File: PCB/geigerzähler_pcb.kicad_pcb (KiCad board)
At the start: 2 copper layers, 155 x 40 mm, 98 parts, among them J1 Molex Micro Fit, J2 Debugpins, J3 USB-TYPE-C-018, J4 Femal Connector for LCD I2C b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, Q1 IRLML6402TRPBF, Q2 BCW68, Q3 PBHV8560Z, Q4 MMBT3904, Q5 MMBT3904, SW1 GPIO4, SW2 GPIO5, SW3 Reset, SW4 Boot, SW5 SW_SPDT, U1 TPS631000DRLR, U2 MCP73871-2AA, U3 ESP32-S3-WROOM-1_multi_unit, U4 ICM7555IBAZ

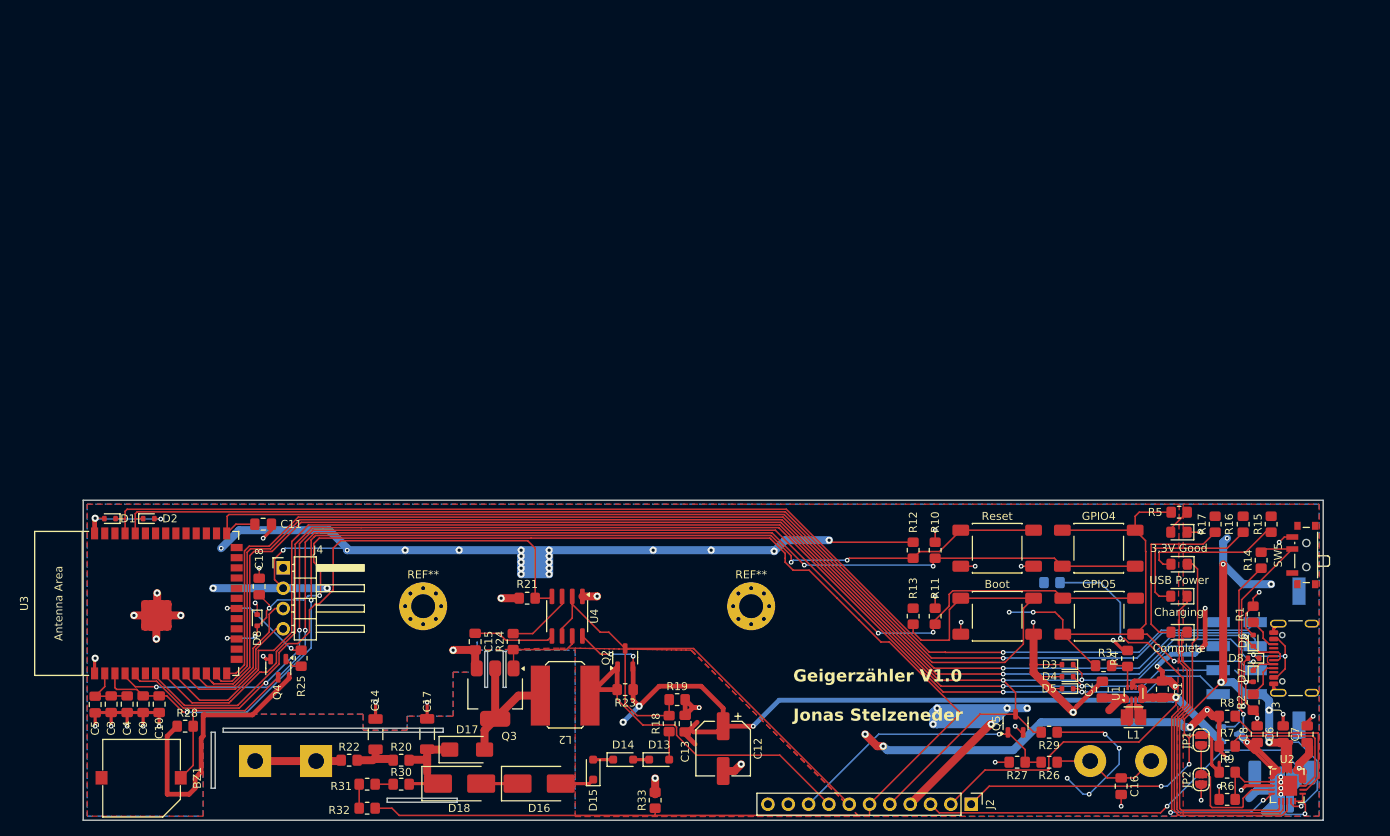
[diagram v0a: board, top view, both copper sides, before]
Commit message: 08.08.2025_v0.2_start
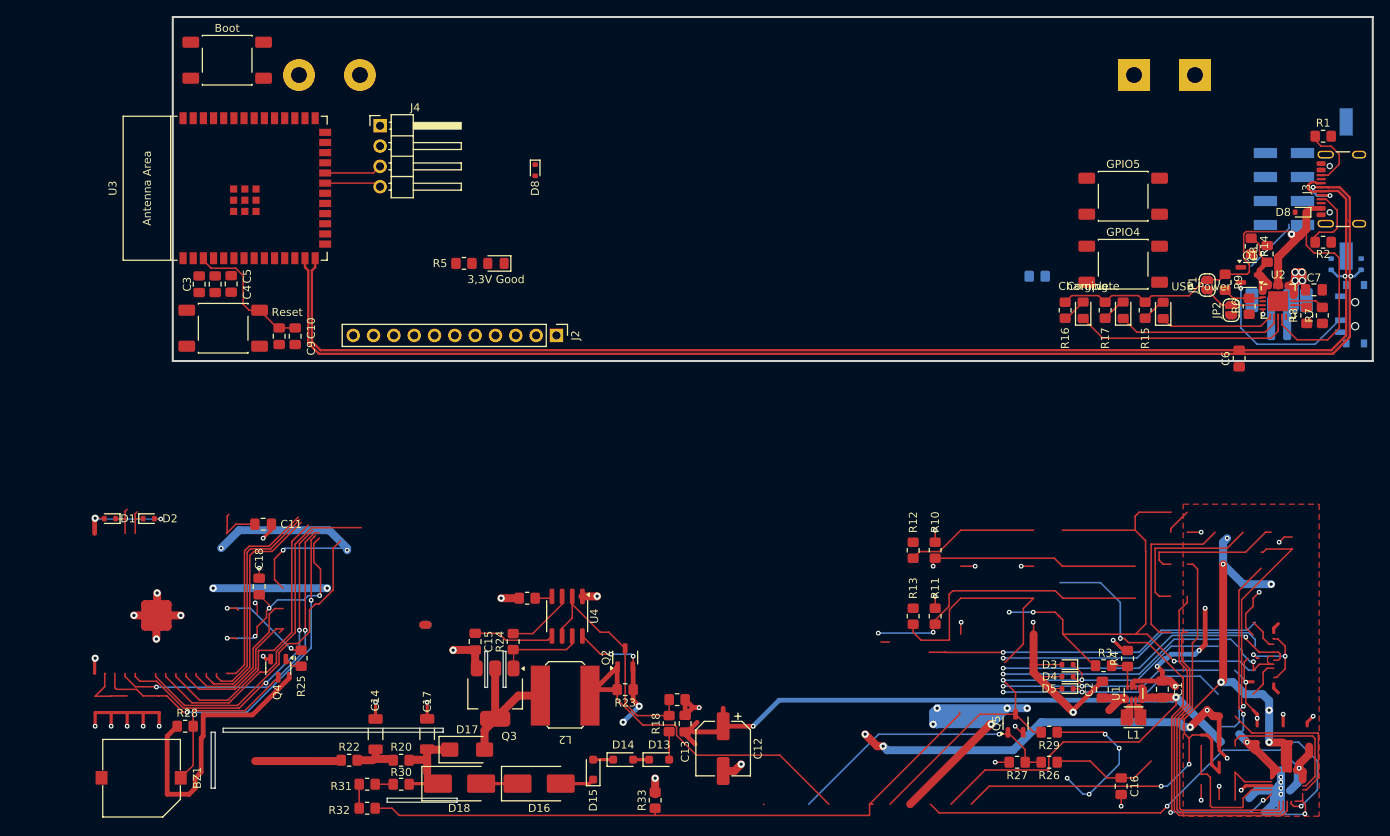
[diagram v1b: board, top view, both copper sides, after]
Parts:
- removed REF** (x2): MountingHole_3mm_Pad_Via, MountingHole:MountingHole_3mm_Pad_Via
- D6, D7, SW5: moved to B.Cu
- Q1: moved to F.Cu
- moved V1 145.4 mm to (209.0, 46.8), turned to 180 degrees
- moved SW4 118.7 mm to (88.0, 45.0)
- moved SW3 100.6 mm to (87.5, 78.5)
- moved R5 94.7 mm to (117.6, 70.4)
- moved D9 91.7 mm to (121.6, 70.4)
- moved J2 78.2 mm to (129.2, 79.4)
- moved D8 66.1 mm to (126.5, 58.8)
- moved R6 61.7 mm to (215.8, 75.8), turned to 90 degrees
- moved R9 61.3 mm to (212.8, 72.8), turned to -90 degrees
- moved U2 60.6 mm to (219.4, 75.1)
- moved R1 60.4 mm to (225.0, 54.5), turned to 0 degrees
- moved C8 60.1 mm to (218.0, 69.2)
- moved BT1 59.1 mm to (219.5, 76.8)
- moved J1 58.9 mm to (220.1, 61.1)
- moved J3 58.9 mm to (228.4, 61.1)
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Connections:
- D3 pad 1: GPIO8 -> GPIO1
- J1 pad 7: GPIO8 -> GPIO1
- Q5 pad 3: GPIO8 -> GPIO1
- R10 pad 1: Net-(U3A-GPIO4) -> Net-(U3A-GPIO10)
- R11 pad 1: Net-(U3A-GPIO5) -> Net-(U3A-GPIO11)
- R21 pad 1: GPIO7 -> GPIO9
- R29 pad 2: GPIO8 -> GPIO1
- SW1 pad 1: Net-(U3A-GPIO4) -> Net-(U3A-GPIO10)
- SW1 pad 3: Net-(U3A-GPIO4) -> Net-(U3A-GPIO10)
- SW2 pad 1: Net-(U3A-GPIO5) -> Net-(U3A-GPIO11)
- SW2 pad 3: Net-(U3A-GPIO5) -> Net-(U3A-GPIO11)
- SW5 pad : (no net) -> GND
- U3 pad 10: I2C_SCL -> unconnected-(U3B-GPIO17/I2C_SCL-Pad10)
- U3 pad 11: I2C_SDA -> unconnected-(U3B-GPIO18/I2C_SDA-Pad11)
- U3 pad 12: GPIO8 -> unconnected-(U3B-GPIO8-Pad12)
- U3 pad 15: unconnected-(U3B-GPIO3/TOUCH3/ADC1_CH2-Pad15) -> Vhigh/100
- U3 pad 17: Vhigh/100 -> GPIO9
- U3 pad 18: unconnected-(U3B-GPIO10/TOUCH10/ADC1_CH9/FSPICS0/FSPIIO4/SUBSPICS0-Pad18) -> Net-(U3A-GPIO10)
- U3 pad 19: unconnected-(U3B-GPIO11/TOUCH11/ADC2_CH0/FSPID/FSPIIO5/SUBSPID-Pad19) -> Net-(U3A-GPIO11)
- U3 pad 21: unconnected-(U3B-GPIO13/TOUCH13/ADC2_CH2/FSPIQ/FSPIIO7/SUBSPIQ-Pad21) -> I2C_SCL
- U3 pad 22: unconnected-(U3B-GPIO14/TOUCH14/ADC2_CH3/FSPIWP/FSPIDQS/SUBSPIWP-Pad22) -> I2C_SDA
- U3 pad 39: unconnected-(U3B-GPIO1-Pad39) -> GPIO1
- U3 pad 4: Net-(U3A-GPIO4) -> unconnected-(U3B-GPIO4-Pad4)
- U3 pad 5: Net-(U3A-GPIO5) -> unconnected-(U3B-GPIO5-Pad5)
- U3 pad 7: GPIO7 -> unconnected-(U3B-GPIO7-Pad7)
- U4 pad 4: GPIO7 -> GPIO9
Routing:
- net GPIO8: track 185.6 -> 29.3 mm, vias 2 -> 0
- net Net-(U3A-GPIO5): track 153.5 -> 0.00 mm, vias 4 -> 0
- net UART0_TX: track 154.3 -> 4.34 mm, vias 1 -> 0
- net Net-(U3A-GPIO4): track 146.1 -> 0.00 mm, vias 4 -> 0
- net (no net): track 0.00 -> 121.4 mm, vias 0 -> 4
- net UART0_RX: track 153.6 -> 37.8 mm
- net Net-(U3A-GPIO0/BOOT): track 141.6 -> 36.9 mm
- net GPIO16/U0CTS: track 159.9 -> 64.7 mm
- net +3.3V: track 325.7 -> 233.7 mm, vias 33 -> 17
- net GPIO15/U0RTS: track 161.2 -> 72.5 mm
- net Vhigh/100: track 196.8 -> 108.2 mm
- net VBUS: track 132.1 -> 212.4 mm, vias 11 -> 13
- net D-: track 164.4 -> 239.1 mm, vias 2 -> 5
- net GPIO7: track 72.2 -> 0.00 mm
- net D+: track 160.2 -> 232.2 mm, vias 2 -> 3
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- removed copper zone on F.Cu, net +3.3V
- removed copper zone on B.Cu, net GND
- removed copper zone on F.Cu, net Vbat_USB
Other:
- board size 155 x 40 mm -> 150 x 98.2 mm
- board text removed: "Geigerzähler V1.0 Jonas Stelzeneder"

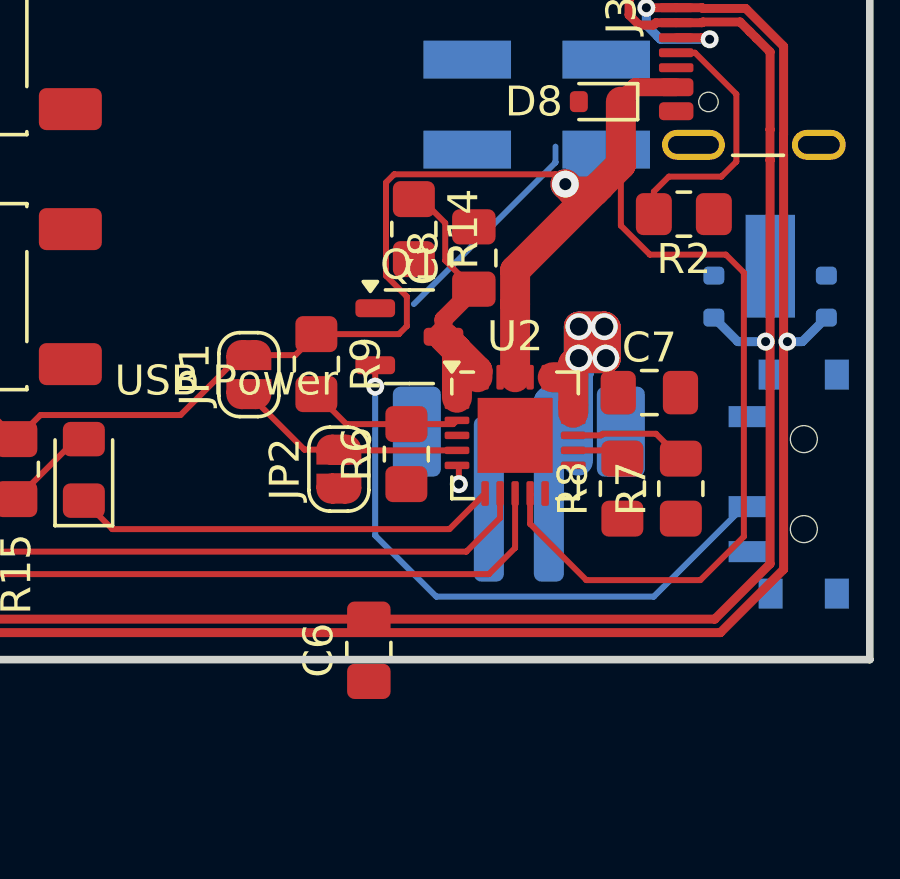
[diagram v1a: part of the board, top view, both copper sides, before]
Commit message: 08.08.2025
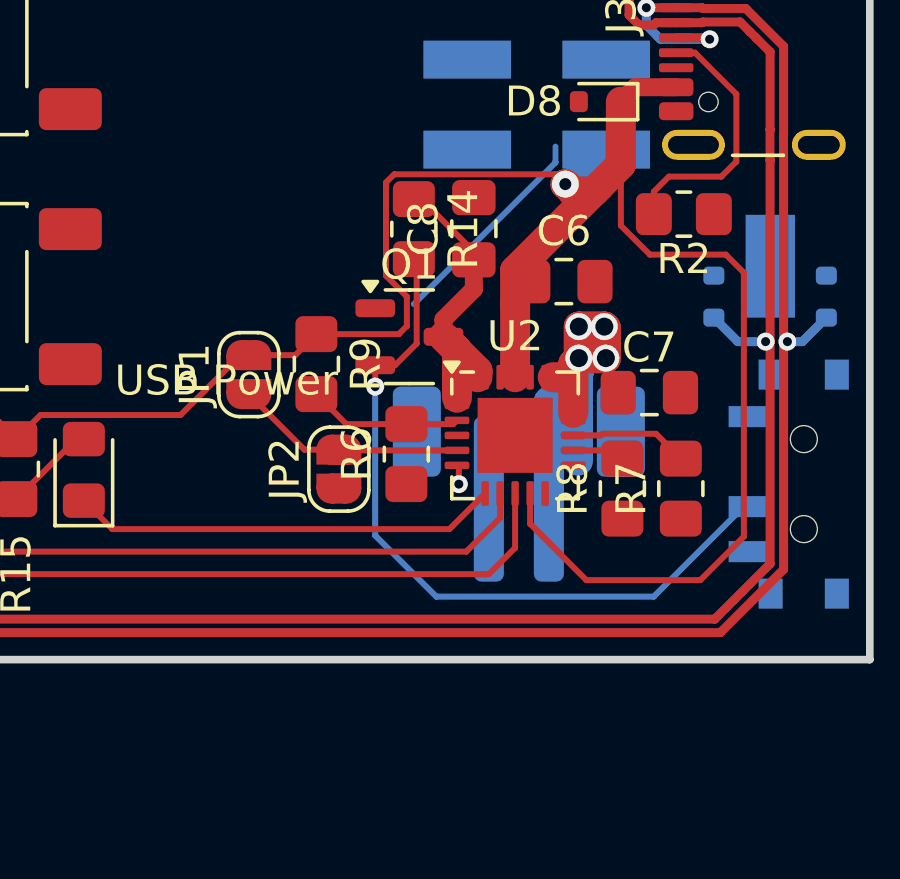
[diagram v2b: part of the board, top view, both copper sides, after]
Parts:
- moved C6 13.9 mm to (221.0, 70.0), turned to 0 degrees
- moved C8 0.98 mm to (218.0, 68.2)
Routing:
- net Net-(Q1-G): track 58.9 -> 63.4 mm
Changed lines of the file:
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@@
 	(footprint "Capacitor_SMD:C_0805_2012Metric_Pad1.18x1.45mm_HandSolder"
 		(layer "F.Cu")
-		(at 218 69.2125 90)
+		(at 218 68.2375 90)
 		(descr "Capacitor SMD 0805 (2012 Metric), square (rectangular) end terminal, IPC-7351 nominal with elongated pad for handsoldering. (Body size source: IPC-SM-782 page 76, https://www.pcb-3d.com/wordpress/wp-content/uploads/ipc-sm-782a_amendment_1_and_2.pdf, https://docs.google.com/spreadsheets/d/1BsfQQcO9C6DZCsRaXUlFlo91Tg2WpOkGARC1WS5S8t0/edit?usp=sharing), generated with kicad-footprint-generator")
 		(tags "capacitor handsolder")
@@
 	(footprint "Capacitor_SMD:C_0805_2012Metric_Pad1.18x1.45mm_HandSolder"
 		(layer "F.Cu")
-		(at 214.5 82.2875 90)
+		(at 221 70)
 		(descr "Capacitor SMD 0805 (2012 Metric), square (rectangular) end terminal, IPC-7351 nominal with elongated pad for handsoldering. (Body size source: IPC-SM-782 page 76, https://www.pcb-3d.com/wordpress/wp-content/uploads/ipc-sm-782a_amendment_1_and_2.pdf, https://docs.google.com/spreadsheets/d/1BsfQQcO9C6DZCsRaXUlFlo91Tg2WpOkGARC1WS5S8t0/edit?usp=sharing), generated with kicad-footprint-generator")
 		(tags "capacitor handsolder")
 		(property "Reference" "C6"
-			(at 0 -1.68 90)
+			(at 0 -1.68 0)
 			(layer "F.SilkS")
 			(effects
@@
 		)
 		(property "Value" "10µF"
-			(at 0 1.68 90)
+			(at 0 1.68 0)
 			(layer "F.Fab")
 			(effects
@@
 		)
 		(property "Datasheet" "https://jlcpcb.com/partdetail/439567-GRM21BR61H106KE43L/C440198"
-			(at 0 0 90)
+			(at 0 0 0)
 			(layer "F.Fab")
 			(hide yes)
@@
 		)
 		(property "Description" "Unpolarized capacitor, small symbol"
-			(at 0 0 90)
+			(at 0 0 0)
 			(layer "F.Fab")
 			(hide yes)
@@
 		)
 		(fp_line
-			(start 1.88 -0.98)
-			(end 1.88 0.98)
+			(start -1.88 -0.98)
+			(end 1.88 -0.98)
 			(stroke
 				(width 0.05)
@@
 		)
 		(fp_line
-			(start -1.88 -0.98)
-			(end 1.88 -0.98)
+			(start -1.88 0.98)
+			(end -1.88 -0.98)
 			(stroke
 				(width 0.05)
@@
 		)
 		(fp_line
-			(start 1.88 0.98)
-			(end -1.88 0.98)
+			(start 1.88 -0.98)
+			(end 1.88 0.98)
 			(stroke
 				(width 0.05)
@@
 		)
 		(fp_line
-			(start -1.88 0.98)
-			(end -1.88 -0.98)
+			(start 1.88 0.98)
+			(end -1.88 0.98)
 			(stroke
 				(width 0.05)
@@
 		)
 		(fp_line
-			(start 1 -0.625)
-			(end 1 0.625)
+			(start -1 -0.625)
+			(end 1 -0.625)
 			(stroke
 				(width 0.1)
@@
 		)
 		(fp_line
-			(start -1 -0.625)
-			(end 1 -0.625)
+			(start -1 0.625)
+			(end -1 -0.625)
 			(stroke
 				(width 0.1)
@@
 		)
 		(fp_line
-			(start 1 0.625)
-			(end -1 0.625)
+			(start 1 -0.625)
+			(end 1 0.625)
 			(stroke
 				(width 0.1)
@@
 		)
 		(fp_line
-			(start -1 0.625)
-			(end -1 -0.625)
+			(start 1 0.625)
+			(end -1 0.625)
 			(stroke
 				(width 0.1)
@@
 		)
 		(fp_text user "${REFERENCE}"
-			(at 0 0 90)
+			(at 0 0 0)
 			(layer "F.Fab")
 			(effects
@@
 		)
 		(pad "1" smd roundrect
-			(at -1.0375 0 90)
+			(at -1.0375 0)
 			(size 1.175 1.45)
 			(layers "F.Cu" "F.Mask" "F.Paste")
@@
 		)
 		(pad "2" smd roundrect
-			(at 1.0375 0 90)
+			(at 1.0375 0)
 			(size 1.175 1.45)
 			(layers "F.Cu" "F.Mask" "F.Paste")
@@
 	)
 	(segment
-		(start 216 67.25)
-		(end 216.25 67.25)
-		(width 0.2)
-		(layer "F.Cu")
-		(net 57)
-	)
-	(segment
 		(start 215.5375 130.2875)
 		(end 215.5 130.25)
@@
 	)
 	(segment
+		(start 216.25 67.25)
+		(end 218 69)
+		(width 0.2)
+		(layer "F.Cu")
+		(net 57)
+	)
+	(segment
 		(start 219.25 133.75)
 		(end 219.5 133.75)
@@
 	)
 	(segment
-		(start 216.25 67.25)
-		(end 217.047 68.047)
+		(start 218 69)
+		(end 218 69.275)
 		(width 0.2)
 		(layer "F.Cu")
@@
 	)
 	(segment
-		(start 217.047 69.297)
-		(end 218 70.25)
-		(width 0.2)
-		(layer "F.Cu")
-		(net 57)
-	)
-	(segment
 		(start 216.9875 71.8375)
 		(end 217.4375 72.2875)
@@
 	)
 	(segment
-		(start 217.047 68.047)
-		(end 217.047 69.297)
-		(width 0.2)
-		(layer "F.Cu")
-		(net 57)
-	)
-	(segment
 		(start 216.9875 71.8375)
 		(end 218.122 72.972)
@@
 	)
 	(segment
+		(start 218 70.25)
+		(end 218 69.275)
+		(width 0.6)
+		(layer "F.Cu")
+		(net 57)
+	)
+	(segment
 		(start 215.5 130.25)
 		(end 216.303 131.053)
@@
 		(net 57)
 	)
+	(segment
+		(start 216 67.25)
+		(end 216.25 67.25)
+		(width 0.2)
+		(layer "F.Cu")
+		(net 57)
+	)
 	(via
 		(at 215.027 126.75)
@@
 	)
 	(segment
+		(start 216.095078 69.345078)
+		(end 216.095078 72.067421)
+		(width 0.2)
+		(layer "F.Cu")
+		(net 58)
+	)
+	(segment
 		(start 214.806 112.434)
 		(end 214.806 125.25)
@@
 	)
 	(segment
+		(start 216.095078 72.067421)
+		(end 215.374999 72.7875)
+		(width 0.2)
+		(layer "F.Cu")
+		(net 58)
+	)
+	(segment
 		(start 214.7125 72.7875)
 		(end 214.7125 73.5)
@@
 	)
 	(segment
+		(start 215.374999 72.7875)
+		(end 214.7125 72.7875)
+		(width 0.2)
+		(layer "F.Cu")
+		(net 58)
+	)
+	(segment
 		(start 216 69.25)
 		(end 216.25 69.25)
 		(width 0.2)
 		(layer "F.Cu")
+		(net 58)
+	)
+	(segment
+		(start 216 69.25)
+		(end 216.095078 69.345078)
+		(width 0.2)
+		(layer "F.Cu")
